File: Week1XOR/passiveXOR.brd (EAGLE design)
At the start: 100 x 80 mm, 27 parts

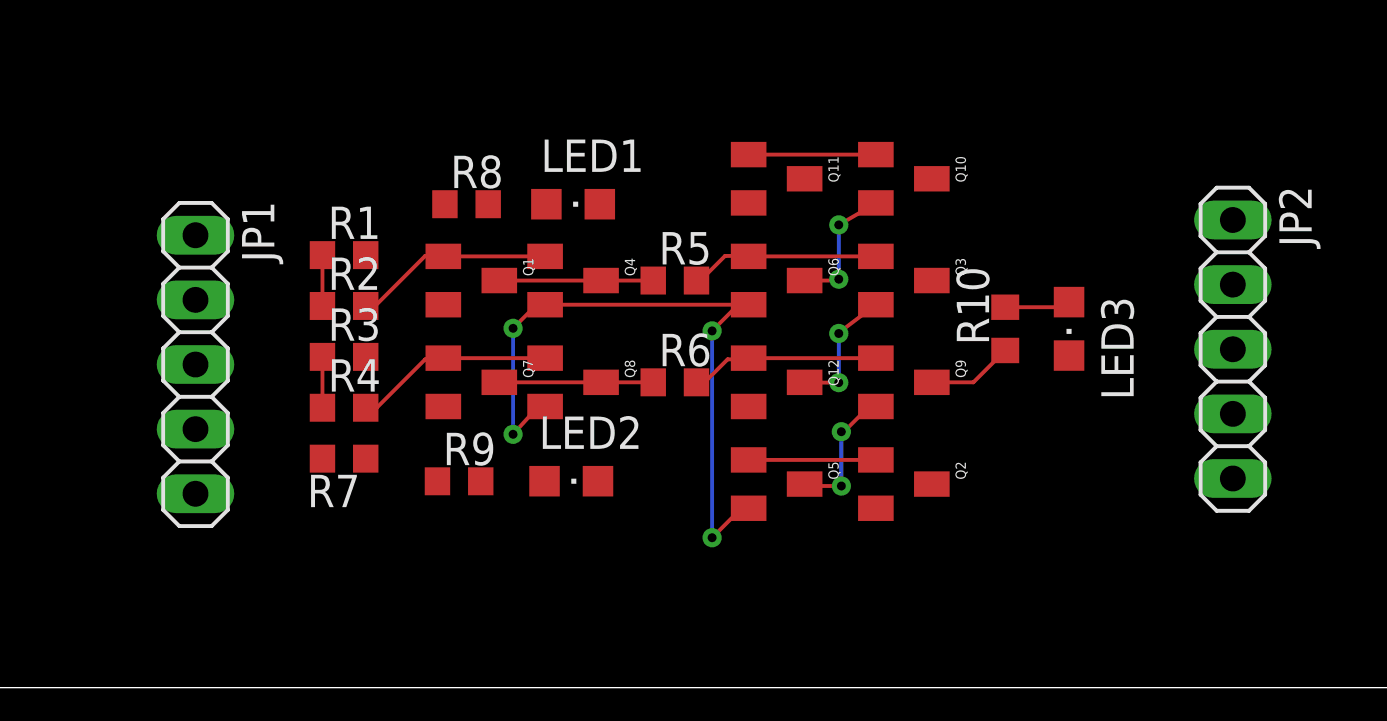
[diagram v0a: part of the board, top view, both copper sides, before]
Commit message: More routing and schmatic fixes
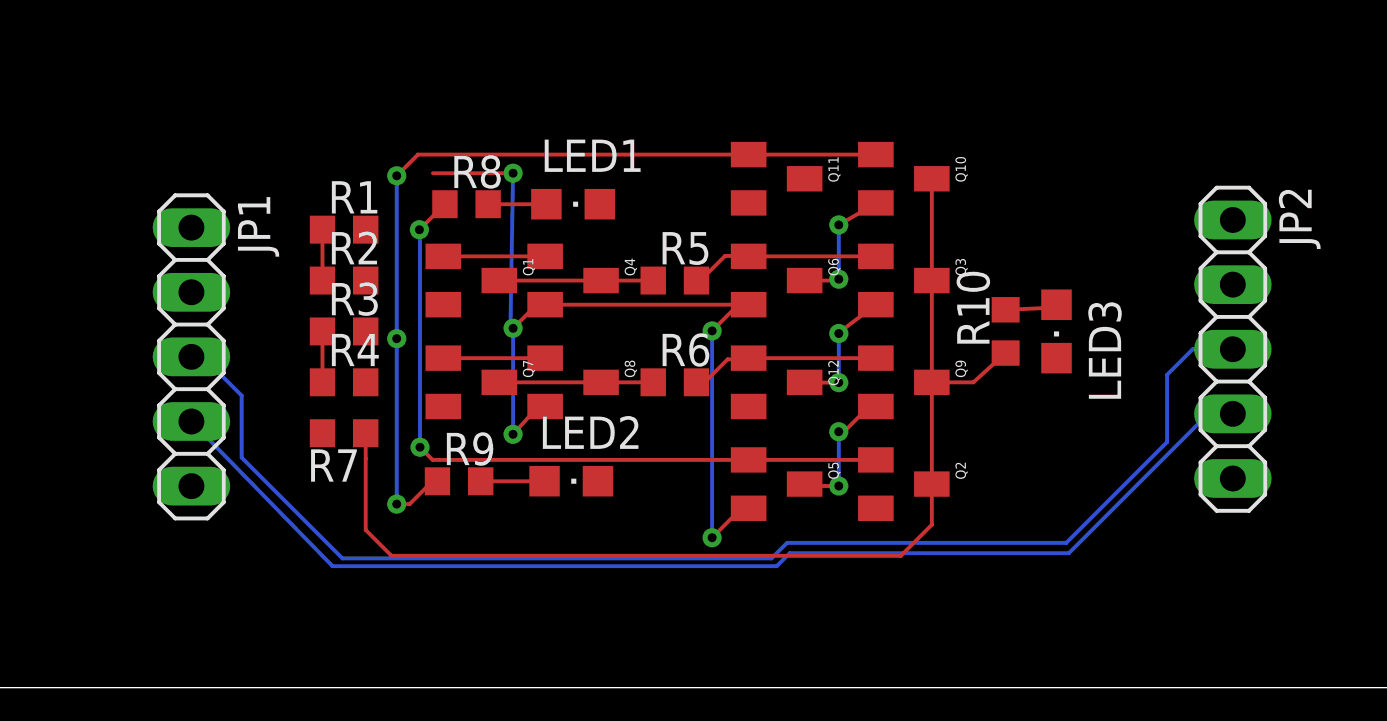
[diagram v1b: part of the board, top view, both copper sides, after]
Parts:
- moved R1 1.00 mm to (15.0, 18.0)
- moved R2 1.00 mm to (15.0, 16.0)
- moved R3 1.00 mm to (15.0, 14.0)
- moved R4 1.00 mm to (15.0, 12.0)
- moved R7 1.00 mm to (15.0, 10.0)
- moved LED3 0.50 mm to (43.0, 14.0)
- moved JP1 0.34 mm to (9.00, 13.0)
- moved R10 0.10 mm to (41.0, 14.0)
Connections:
- removed net VCC: JP1.1, JP2.1
- net A: no longer JP2.2
- net B: no longer JP2.3
- net C: no longer JP2.4
- net INA: now also JP2.2
- net INB: now also JP2.3
- net OUTC: now also JP2.4
- net VDD: now also JP1.1, JP2.1
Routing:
- net INB: track 2.00 -> 52.5 mm
- net OUTC: track 0.00 -> 45.8 mm
- net C: track 3.40 -> 43.9 mm
- net B: track 5.00 -> 34.2 mm, vias 0 -> 3
- net A: track 5.00 -> 28.1 mm, vias 0 -> 2
- net VDD: track 27.5 -> 36.7 mm, vias 4 -> 5
- net NOT1A: track 7.87 -> 4.00 mm
- net NOT2A: track 7.86 -> 4.00 mm
- net N$4: track 0.00 -> 2.51 mm
- net N$1: track 0.00 -> 2.29 mm

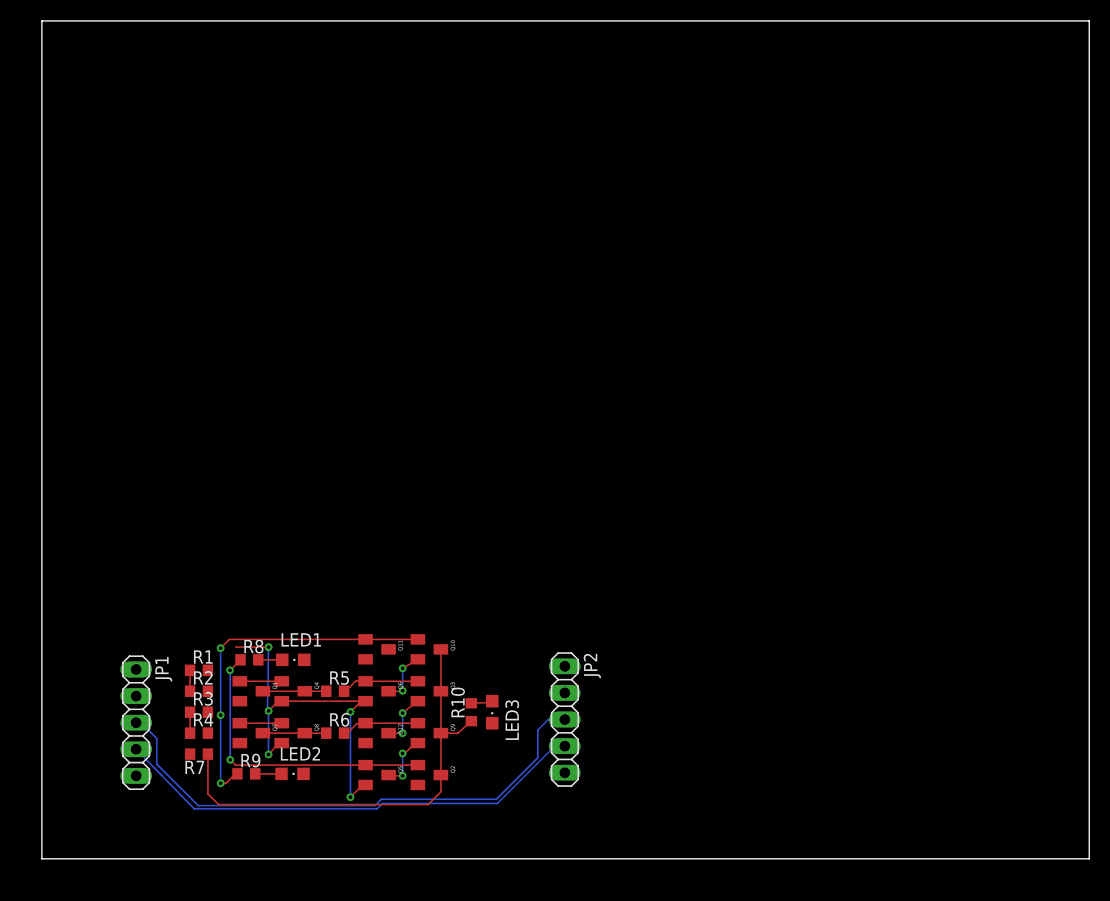
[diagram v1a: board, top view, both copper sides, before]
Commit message: More routing Tweaking and started to make pretty
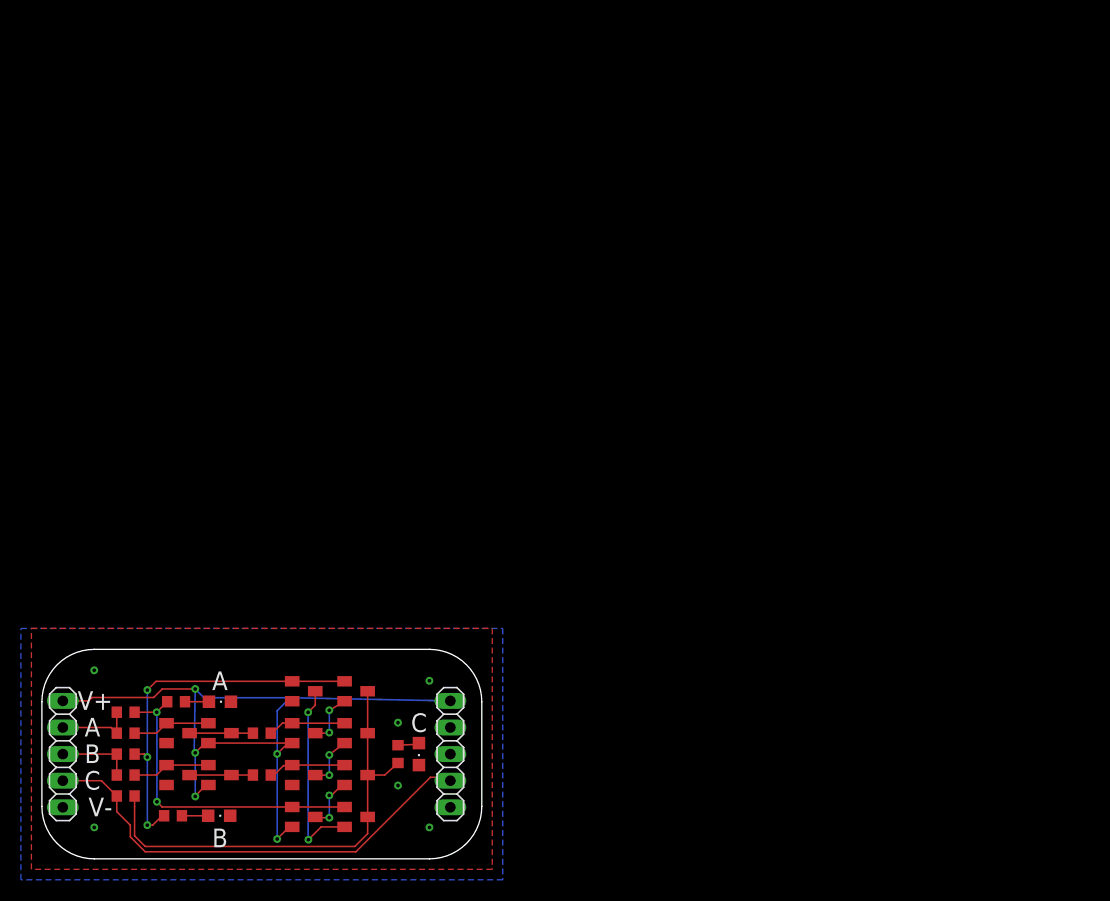
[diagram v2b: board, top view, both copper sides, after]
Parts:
- moved JP2 11.4 mm to (39.0, 10.0)
- moved LED1 8.06 mm to (17.0, 15.0)
- moved LED2 8.06 mm to (16.9, 4.11)
- moved LED3 8.06 mm to (36.0, 10.0)
- moved Q1 8.06 mm to (13.0, 12.0)
- moved Q10 8.06 mm to (30.0, 16.0)
- moved Q11 8.06 mm to (25.0, 16.0)
- moved Q12 8.06 mm to (25.0, 8.00)
- moved Q2 8.06 mm to (30.0, 4.00)
- moved Q3 8.06 mm to (30.0, 12.0)
- moved Q4 8.06 mm to (17.0, 12.0)
- moved Q5 8.06 mm to (25.0, 4.00)
- moved Q6 8.06 mm to (25.0, 12.0)
- moved Q7 8.06 mm to (13.0, 8.00)
- moved Q8 8.06 mm to (17.0, 8.00)
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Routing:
- net INB: track 52.5 -> 7.15 mm
- net VDD: track 36.7 -> 77.3 mm
- net N$20: track 0.00 -> 18.5 mm, vias 0 -> 2
- net INA: track 2.00 -> 7.37 mm
- net NOT2A: track 4.00 -> 7.44 mm
- net NOT1A: track 4.00 -> 7.44 mm
- net A: track 28.1 -> 30.2 mm
- net B: track 34.2 -> 35.5 mm
- added copper zone on layer 1, net GND
- added copper zone on layer 16, net GND
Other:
- board size 100 x 80 mm -> 42 x 20 mm
- board text added: "A"
- board text added: "B"
- board text added: "C"
- board text added: "V+"
- board text added: "V-"
